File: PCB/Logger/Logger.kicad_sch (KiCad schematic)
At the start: 23 parts, among them J2 USB-C-Socket-V, J3 USB-PROG, J5 Conn_01x05, J5 POWER, J6 DM3AT-SF-PEJM5, J8 Shelly, U1 MD8942, U10 ESP32-S3-MINI-1, U5 QR

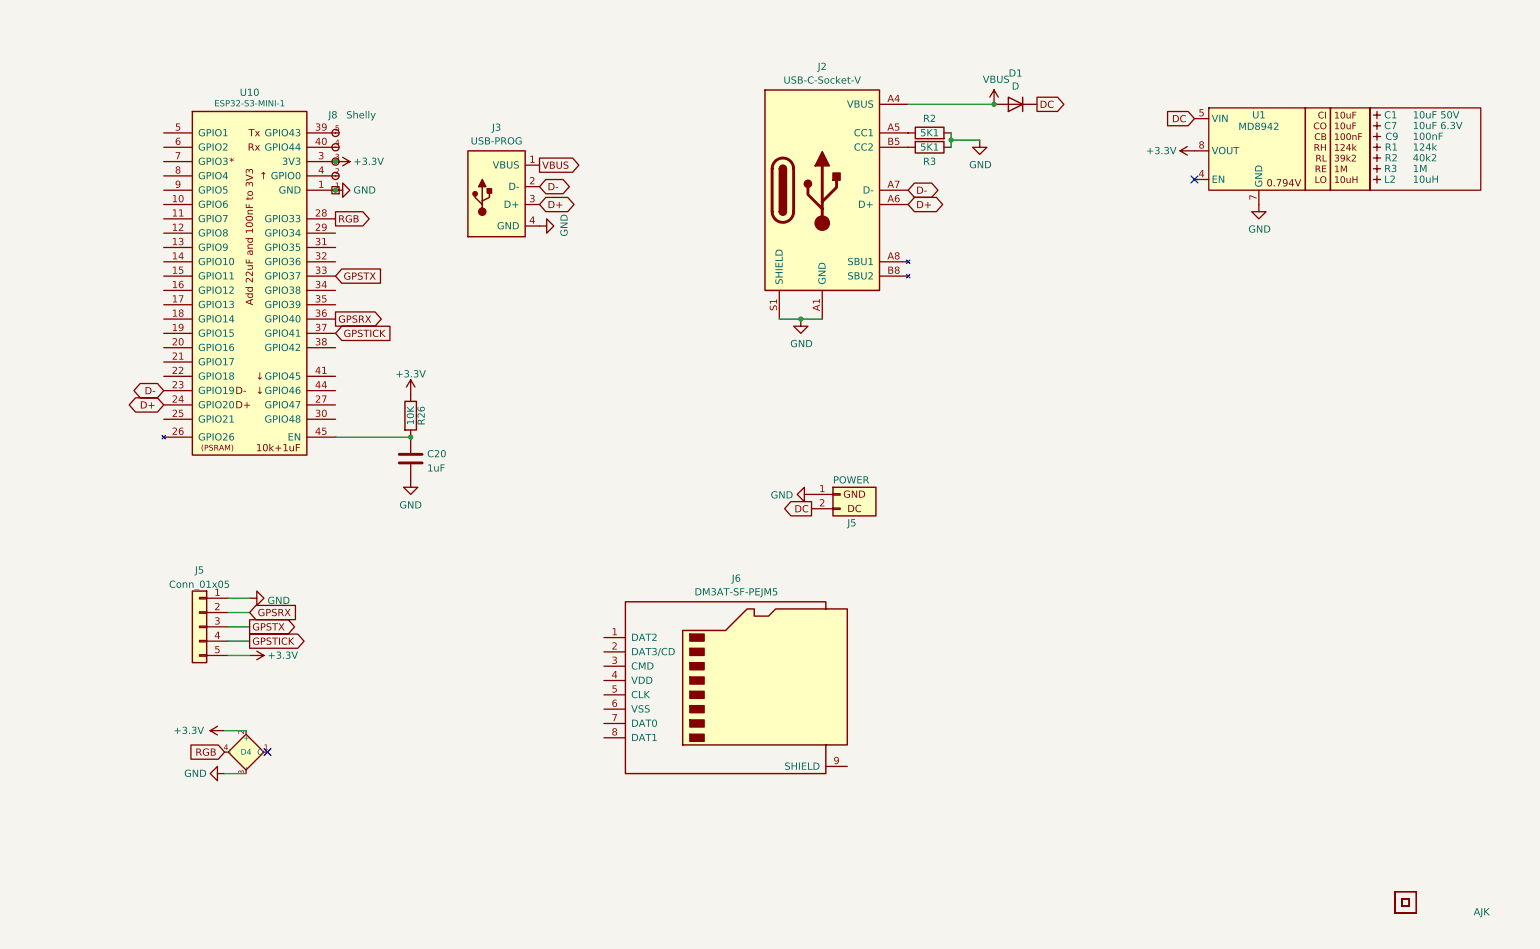
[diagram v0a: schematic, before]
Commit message: More work
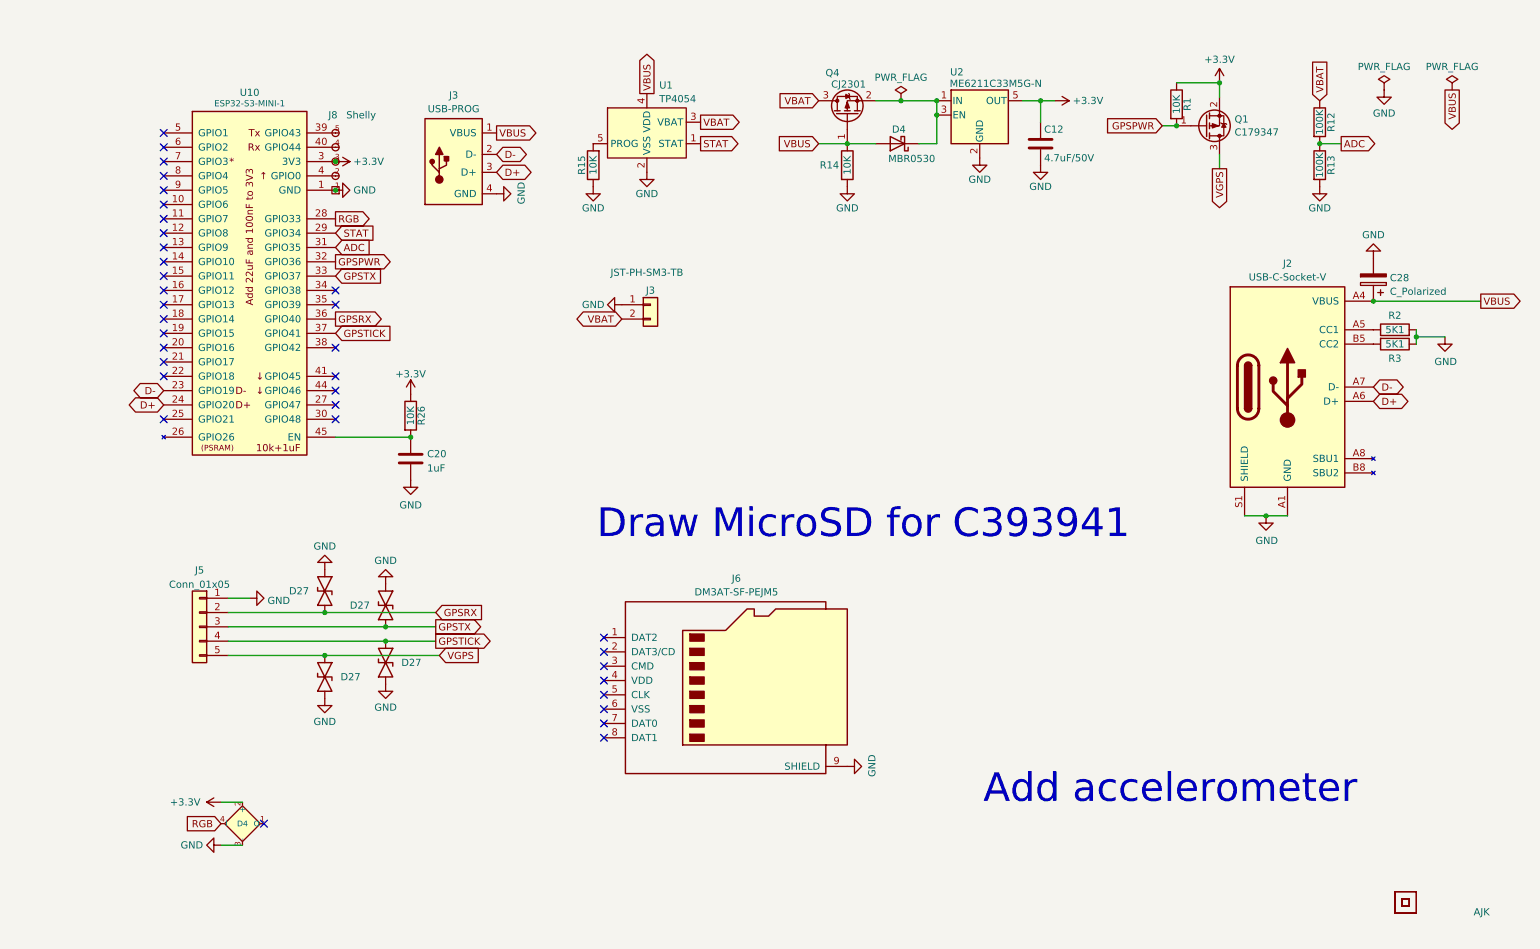
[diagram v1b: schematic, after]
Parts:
- removed C1: 10uF 50V, RevK:C_0603_, symbol RevK:Hidden
- removed C7: 10uF 6.3V, RevK:C_0603_, symbol RevK:Hidden
- removed C9: 100nF, RevK:C_0603_, symbol RevK:Hidden
- removed D1: D, RevK:D_1206, symbol Device:D
- removed J5: POWER, RevK:PTSM-HH1-2-RA, symbol RevK:PowerIn
- removed L2: 10uH, RevK:L_4x4_, symbol RevK:Hidden
- removed R1: 124k, RevK:R_0402_, symbol RevK:Hidden
- removed R2: 40k2, RevK:R_0402_, symbol RevK:Hidden
- removed R3: 1M, RevK:R_0402_, symbol RevK:Hidden
- removed U1: MD8942, RevK:SOT-23-6-MD8942, symbol RevK:MD89420-RegBlock
- added C12: 4.7uF/50V, RevK:C_0805, symbol Device:C
- added C28: C_Polarized, Capacitor_Tantalum_SMD:CP_EIA-7343-31_Kemet-D, symbol Device:C_Polarized
- added D27 (x4): ~, RevK:DFN1006-2L, symbol RevK:ES05D1MC10
- added D4: MBR0530, RevK:D_SOD-123, symbol Device:D_Schottky
- added J3: JST-PH-SM3-TB, Connector_JST:JST_PH_S2B-PH-SM4-TB_1x02-1MP_P2.00mm_Horizontal, symbol Connector_Generic:Conn_01x02
- added Q1: C179347, RevK:SOT-323_SC-70, symbol Device:Q_PMOS_GSD
- added Q4: CJ2301, RevK:SOT-23, symbol Transistor_FET:BSS83P
- added R1, R14, R15: 10K, RevK:R_0402, symbol Device:R
- added R12, R13: 100K, RevK:R_0402, symbol Device:R
- added U1: TP4054, RevK:SOT-23-5, symbol RevK:TP4054
- added U2: ME6211C33M5G-N, RevK:SOT-23-5, symbol Regulator_Linear:TLV70033_SOT23-5
- J5: now left out of the parts list
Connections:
- net GND: now also J6.9 (SHIELD), C12.2, C28.2, D27.1, D27.1, D27.1, D27.1, J3.1 (Pin_1), R13.2, R14.2, R15.1, U1.2 (VSS), U2.2 (GND)
- net GPSRX: now also D27.2
- net GPSTICK: now also D27.2
- net GPSTX: now also D27.2
- net VBUS: now also C28.1, D4.2 (A), Q4.1 (G), R14.1, U1.4 (VDD)
- net STAT: now reaches U10.29 (GPIO34)
- net STAT: now also U1.1 (STAT)
- net ADC: now reaches U10.31 (GPIO35)
- net ADC: now also R12.2, R13.1
- net GPSPWR: now reaches U10.32 (GPIO36)
- net GPSPWR: now also Q1.1 (G), R1.2
- net +3V3 renamed +3.3V
- net +3.3V: now also C12.1, Q1.2 (S), R1.1, U2.5 (OUT); no longer J5.5 (Pin_5)
- new net: D4.1 (K), Q4.2 (S), U2.1 (IN), U2.3 (EN)
- new net: R15.2, U1.5 (PROG)
- new net VBAT: J3.2 (Pin_2), Q4.3 (D), R12.1, U1.3 (VBAT)
- new net VGPS: D27.2, J5.5 (Pin_5), Q1.3 (D)
- no-connect marks 2 -> 35
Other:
- note added: "Add accelerometer"
- note added: "Draw MicroSD for C393941"
- moved on the sheet: D4, J2, J3, R2, R3

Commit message: Ready to order
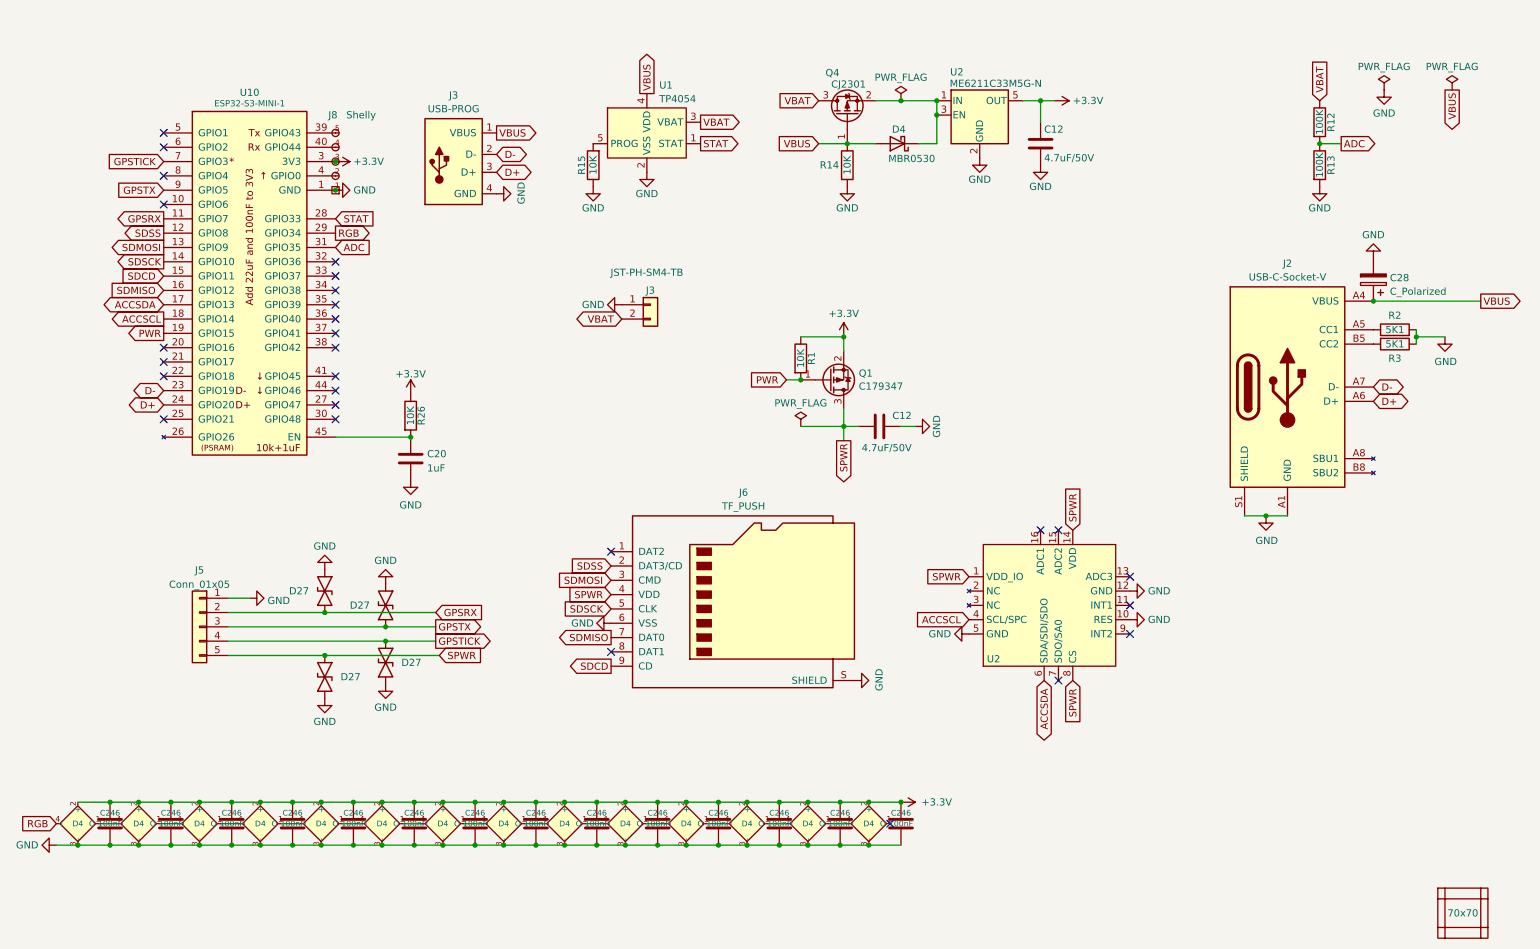
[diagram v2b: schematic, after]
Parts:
- removed J6: DM3AT-SF-PEJM5, Connector_Card:microSD_HC_Hirose_DM3AT-SF-PEJM5, symbol Connector:Micro_SD_Card
- removed Logo2: AJK, RevK:AJK, symbol RevK:AJK
- removed U5: QR, RevK:QR-SS, symbol RevK:QR
- added C12: 4.7uF/50V, RevK:C_0805, symbol Device:C
- added C246 (x14): 100nF, RevK:C_0402, symbol Device:C
- added D4 (x13): XL-1010RGBC-WS2812B, RevK:SMD1010, symbol RevK:WS2812B-1mm
- added J6: TF_PUSH, RevK:TF_PUSH, symbol RevK:TF_PUSH
- added PCB1: 70x70, RevK:PCB7070, symbol RevK:PCB
- added U2: ~, Package_LGA:LGA-16_3x3mm_P0.5mm_LayoutBorder3x5y, symbol RevK:LIS3DHTR
- added V1, V3, V4, V6: ~, RevK:VCUT70N, symbol RevK:VCUT
- J3: value JST-PH-SM3-TB -> JST-PH-SM4-TB; footprint Connector_JST:JST_PH_S2B-PH-SM4-TB_1x02-1MP_P2.00mm_Horizontal -> RevK:JST_PH_S2B-PH-SM4-TB_1x02-1MP_P2.00mm_Horizontal
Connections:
- net +3.3V: now also C246.1, C246.1, C246.1, C246.1, C246.1, C246.1, C246.1, C246.1, C246.1, C246.1, C246.1, C246.1, C246.1, C246.1, D4.2 (+), D4.2 (+), D4.2 (+), D4.2 (+), D4.2 (+), D4.2 (+), D4.2 (+), D4.2 (+), D4.2 (+), D4.2 (+), D4.2 (+), D4.2 (+), D4.2 (+)
- net GND: now also C12.2, C246.2, C246.2, C246.2, C246.2, C246.2, C246.2, C246.2, C246.2, C246.2, C246.2, C246.2, C246.2, C246.2, C246.2, D4.3 (-), D4.3 (-), D4.3 (-), D4.3 (-), D4.3 (-), D4.3 (-), D4.3 (-), D4.3 (-), D4.3 (-), D4.3 (-), D4.3 (-), D4.3 (-), D4.3 (-), J6.6 (VSS), J6.S (SHIELD), U2.10 (RES), U2.12 (GND), U2.5 (GND)
- net GPSRX: now also U10.11 (GPIO7); no longer U10.36 (GPIO40)
- net GPSTICK: now also U10.7 (GPIO3); no longer U10.37 (GPIO41)
- net GPSTX: now also U10.9 (GPIO5); no longer U10.33 (GPIO37)
- net RGB: now also U10.29 (GPIO34); no longer U10.28 (GPIO33)
- net STAT: now also U10.28 (GPIO33); no longer U10.29 (GPIO34)
- net at D4.1 (O): now also D4.4 (I)
- net SDSS: now reaches U10.12 (GPIO8)
- net SDSS: now also J6.2 (DAT3/CD)
- net SDMOSI: now reaches U10.13 (GPIO9)
- net SDMOSI: now also J6.3 (CMD)
- net SDSCK: now reaches U10.14 (GPIO10)
- net SDSCK: now also J6.5 (CLK)
- net SDCD: now reaches U10.15 (GPIO11)
- net SDCD: now also J6.9 (CD)
- net SDMISO: now reaches U10.16 (GPIO12)
- net SDMISO: now also J6.7 (DAT0)
- net ACCSDA: now reaches U10.17 (GPIO13)
- net ACCSDA: now also U2.6 (SDA/SDI/SDO)
- net ACCSCL: now reaches U10.18 (GPIO14)
- net ACCSCL: now also U2.4 (SCL/SPC)
- net PWR: now reaches U10.19 (GPIO15)
- net PWR: now also Q1.1 (G), R1.2
- removed net GPSPWR: Q1.1 (G), R1.2, U10.32 (GPIO36)
- net VGPS renamed SPWR
- net SPWR: now also C12.1, J6.4 (VDD), U2.1 (VDD_IO), U2.14 (VDD), U2.8 (CS)
- new net: D4.1 (O), D4.4 (I) (x12)
- no-connect marks 35 -> 28
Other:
- note removed: "Add accelerometer"
- note removed: "Draw MicroSD for C393941"
- moved on the sheet: D4, Q1, R1

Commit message: Ready to order
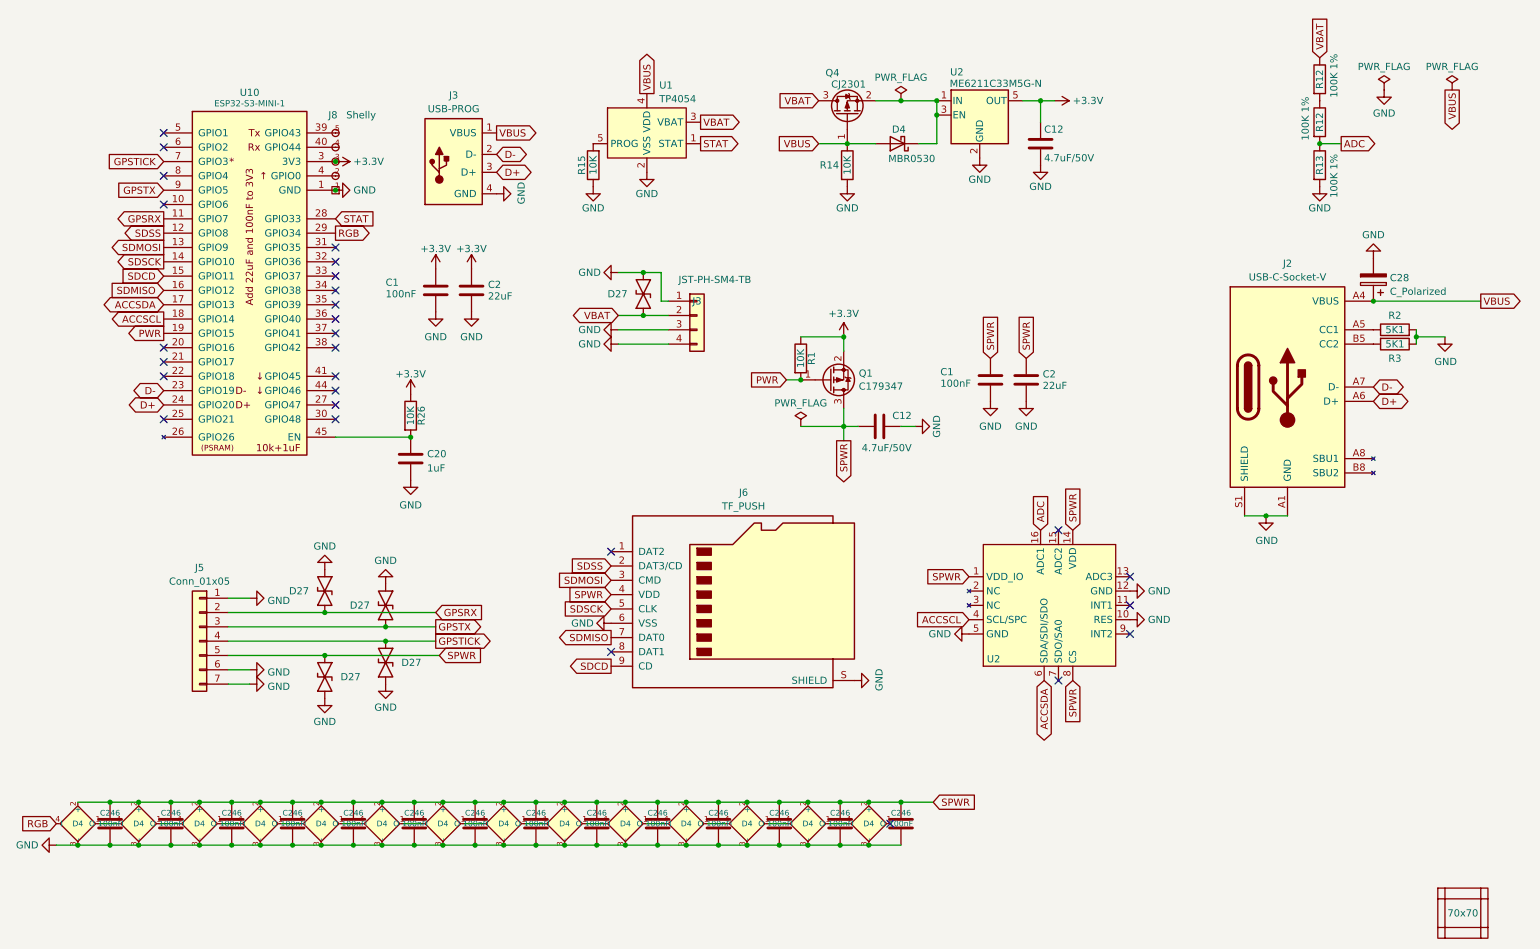
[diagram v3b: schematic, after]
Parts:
- added C1 (x2): 100nF, RevK:C_0402, symbol Device:C
- added C2 (x2): 22uF, RevK:C_0603, symbol Device:C
- added D27: ~, RevK:DFN1006-2L, symbol RevK:ES05D1MC10
- added R12: 100K 1%, RevK:R_0402, symbol Device:R
- J3: symbol Connector_Generic:Conn_01x02 -> Connector_Generic:Conn_01x04
- J5: symbol Connector_Generic:Conn_01x05 -> Connector_Generic:Conn_01x07; now in the parts list
- R12, R13: value 100K -> 100K 1%
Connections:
- net +3.3V: now also C1.1, C2.1; no longer C246.1, C246.1, C246.1, C246.1, C246.1, C246.1, C246.1, C246.1, C246.1, C246.1, C246.1, C246.1, C246.1, C246.1, D4.2 (+), D4.2 (+), D4.2 (+), D4.2 (+), D4.2 (+), D4.2 (+), D4.2 (+), D4.2 (+), D4.2 (+), D4.2 (+), D4.2 (+), D4.2 (+), D4.2 (+), D4.2 (+)
- net ADC: now also U2.16 (ADC1); no longer U10.31 (GPIO35)
- net GND: now also J3.3 (Pin_3), J3.4 (Pin_4), J5.6 (Pin_6), J5.7 (Pin_7), C1.2, C1.2, C2.2, C2.2, D27.1
- net SPWR: now also C246.1, C246.1, C246.1, C246.1, C246.1, C246.1, C246.1, C246.1, C246.1, C246.1, C246.1, C246.1, C246.1, C246.1, D4.2 (+), D4.2 (+), D4.2 (+), D4.2 (+), D4.2 (+), D4.2 (+), D4.2 (+), D4.2 (+), D4.2 (+), D4.2 (+), D4.2 (+), D4.2 (+), D4.2 (+), D4.2 (+), C1.1, C2.1
- net VBAT: now also D27.2, R12.1; no longer R12.1
- new net: R12.1, R12.2

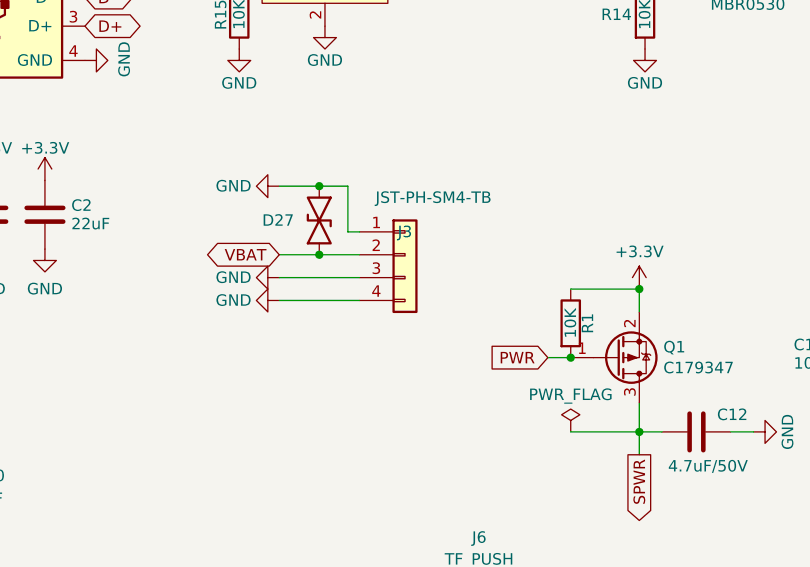
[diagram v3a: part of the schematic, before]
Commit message: Ordered
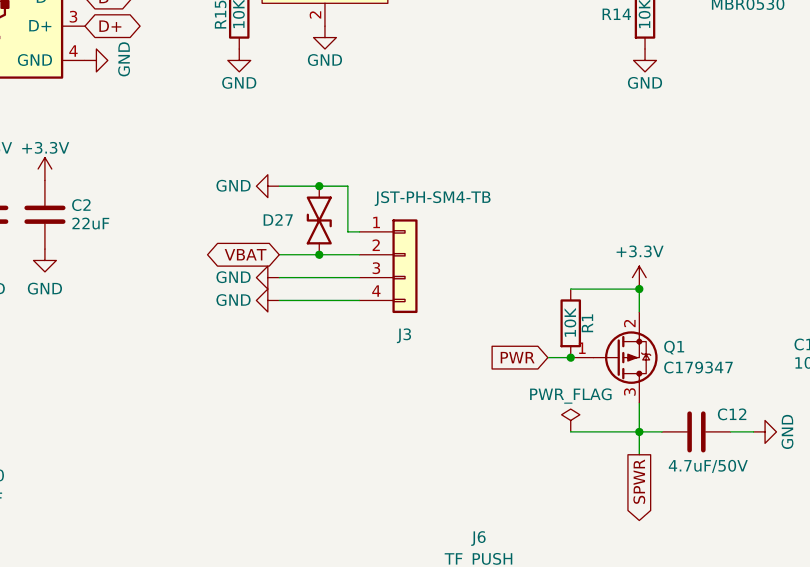
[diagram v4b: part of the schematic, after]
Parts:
- J5: now left out of the parts list
- R12, R13: LCSC Part # (none) -> C5139597
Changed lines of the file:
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@@
       (effects (font (size 1.27 1.27)) hide)
     )
+    (property "LCSC Part #" "C5139597" (at 247.65 41.275 90)
+      (effects (font (size 1.27 1.27)) hide)
+    )
     (pin "1")
     (pin "2")
@@
   )
   (symbol (lib_id "Connector_Generic:Conn_01x07") (at 48.895 125.73 0) (mirror y) (unit 1)
-    (in_bom yes) (on_board yes) (dnp no) (fields_autoplaced)
+    (in_bom no) (on_board yes) (dnp no) (fields_autoplaced)
     (property "Reference" "J5" (at 48.895 112.6957 0)
       (effects (font (size 1.27 1.27)))
@@
       (effects (font (size 1.27 1.27)) hide)
     )
+    (property "LCSC Part #" "C5139597" (at 247.65 33.655 90)
+      (effects (font (size 1.27 1.27)) hide)
+    )
     (pin "1")
     (pin "2")
@@
       (effects (font (size 1.27 1.27)) hide)
     )
+    (property "LCSC Part #" "C5139597" (at 247.65 26.035 90)
+      (effects (font (size 1.27 1.27)) hide)
+    )
     (pin "1")
     (pin "2")
@@
   (symbol (lib_id "Connector_Generic:Conn_01x04") (at 137.16 67.945 0) (unit 1)
     (in_bom yes) (on_board yes) (dnp no)
-    (property "Reference" "J3" (at 137.16 65.405 0)
+    (property "Reference" "J3" (at 137.16 76.835 0)
       (effects (font (size 1.27 1.27)))
     )
